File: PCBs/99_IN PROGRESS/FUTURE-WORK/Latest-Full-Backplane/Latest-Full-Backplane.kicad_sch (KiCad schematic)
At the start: 0 parts

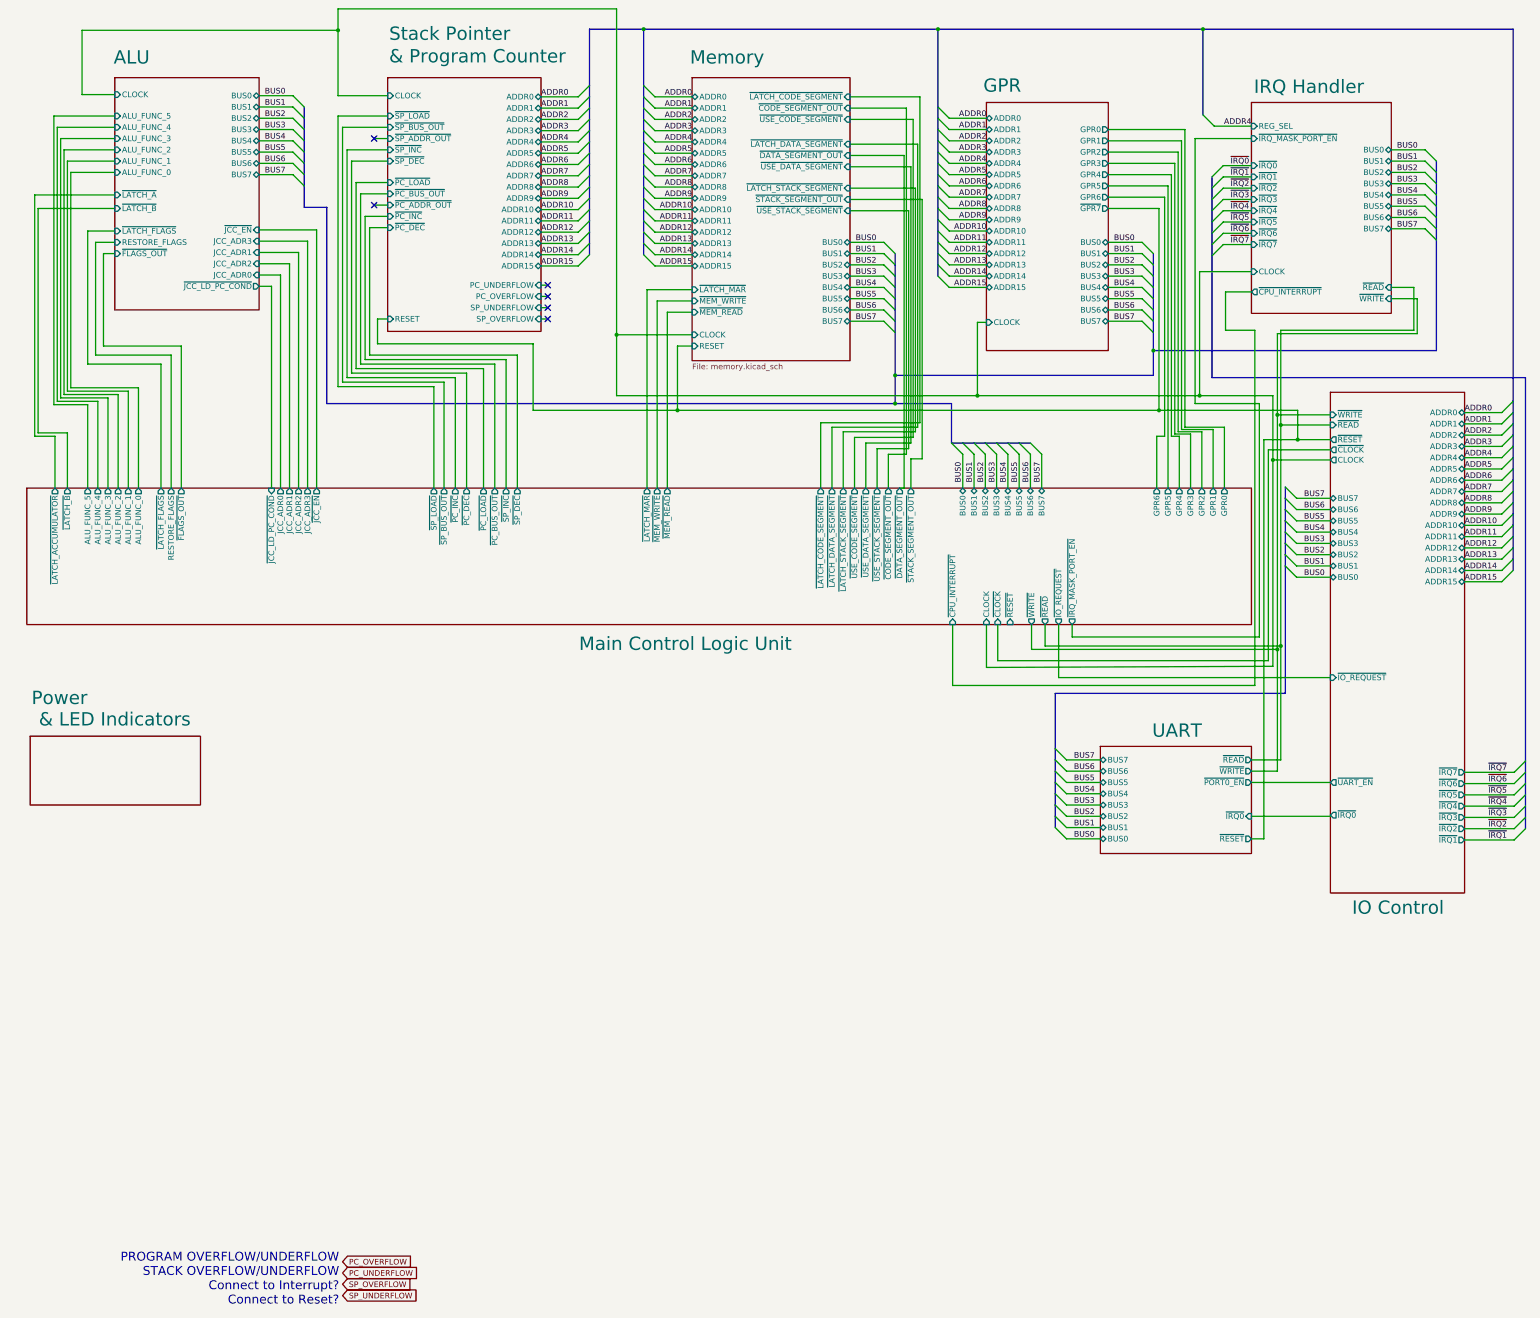
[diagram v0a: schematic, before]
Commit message: cray cray save
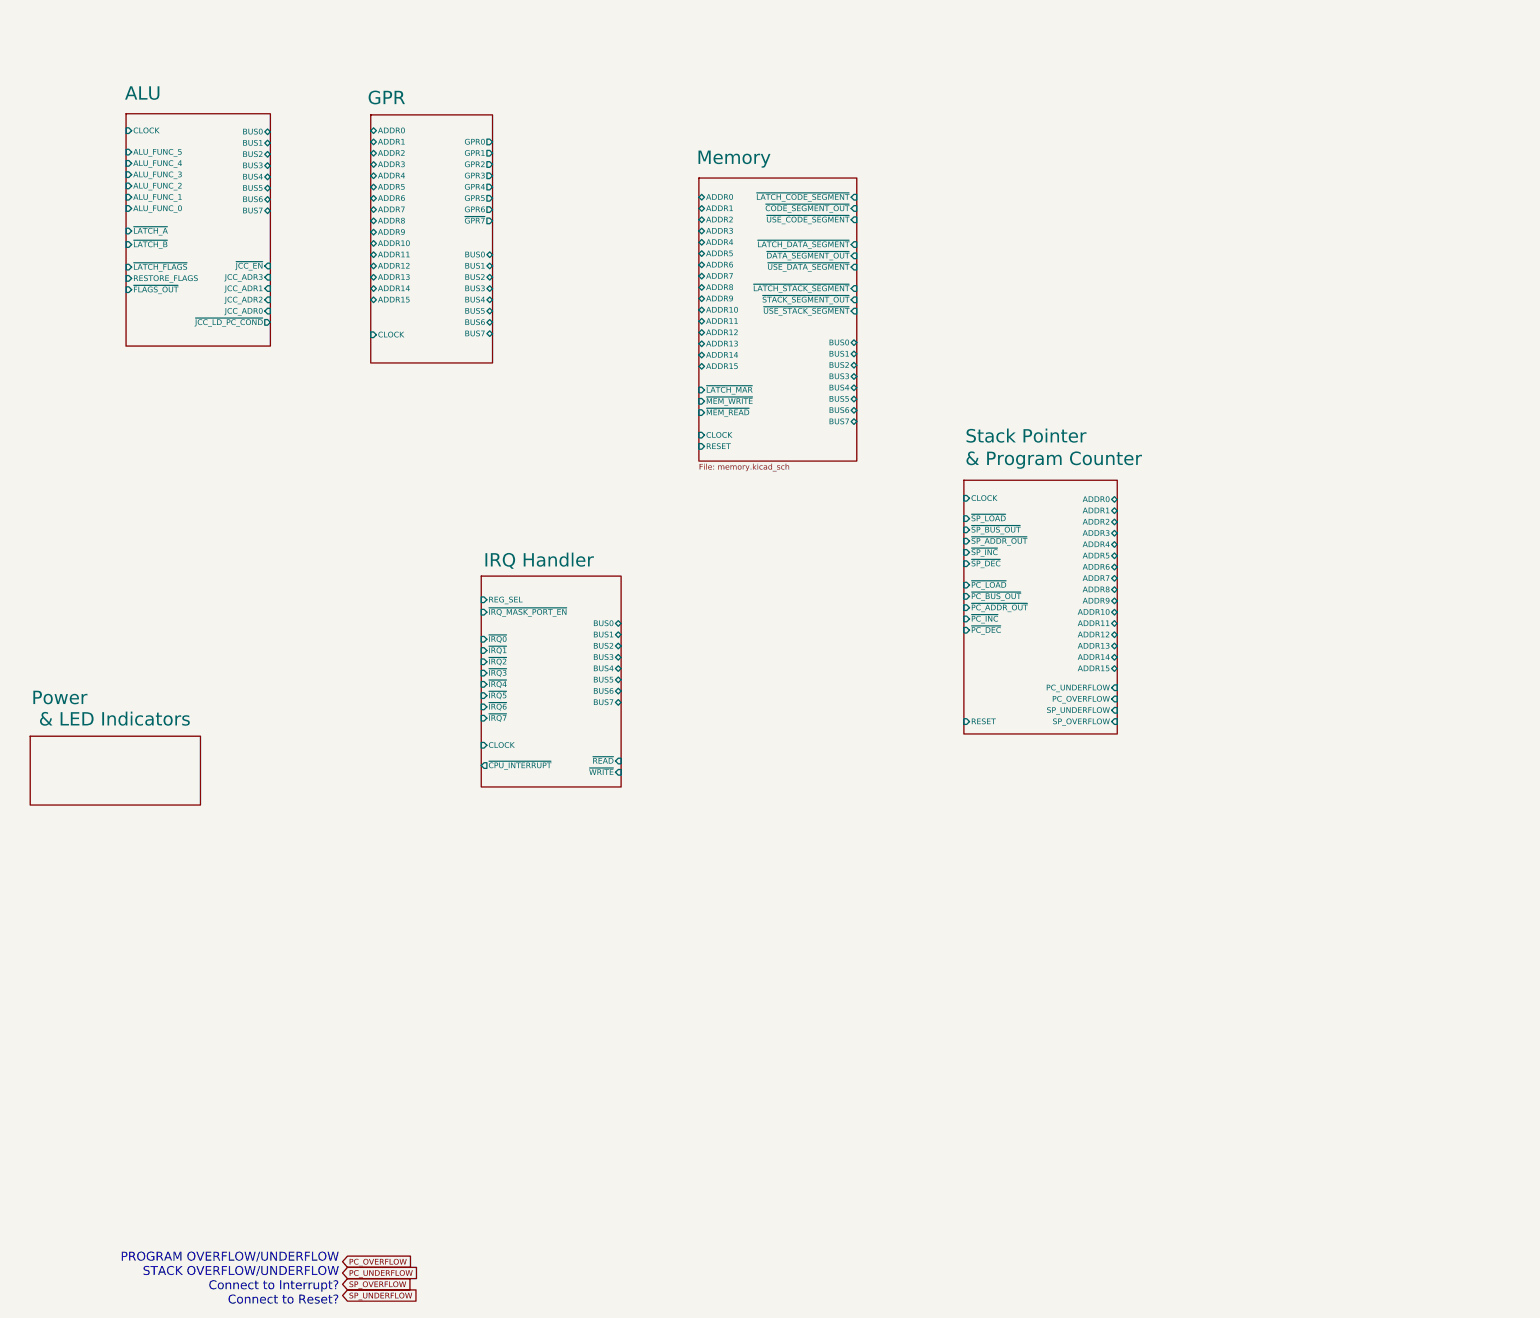
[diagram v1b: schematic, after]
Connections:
- no-connect marks 6 -> 0
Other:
- removed sheet Control Unit
- removed sheet IO Control
- removed sheet uart
